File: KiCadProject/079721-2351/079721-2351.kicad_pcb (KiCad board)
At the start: 2 copper layers, 159.3 x 154.2 mm, 241 parts, among them IC1 HC244, IC101 uPC177C, IC201 MP493, IC401 D151811-0360, IC402 IS157, IC501 D151821-0020, IC601 MP5273, J201 Connected, J44 Conn_02x11_0x13_Top_Bottom_Sh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, J601 Connected, J711 Empty, Q802 C945, T1 2SB1015B, T211 RN1006, T711 2CS2001, T712A1 2SD1415, T721 2CS2001, T722A1 2SD1415, T751 CE1A3Q, T761 CE1A3Q, T801 2CS2001, T803 2CS4065, T811 2SC1815, T812 CE1A3Q, T821 Empty, T822 CE1A3Q (empty), T831 Empty, T832 CE1A3Q (empty), T841 2CS2001, T842 CE1A3Q, T851 Empty, T852 CE1A3Q (empty), T861 Empty, T911 RN1006, T921 RN1006, T921A1 Conn_01x01_Female, T921B1 Conn_01x01_Female, U1 4071, U2 4069, X601 Crystal

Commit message: Cleanup
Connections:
- net IC402_24 renamed IC401_24
- net Net-(C491-Pad2) renamed IC401_19
- net Vehicle_speed_sensor renamed Transsmision_control_module_2

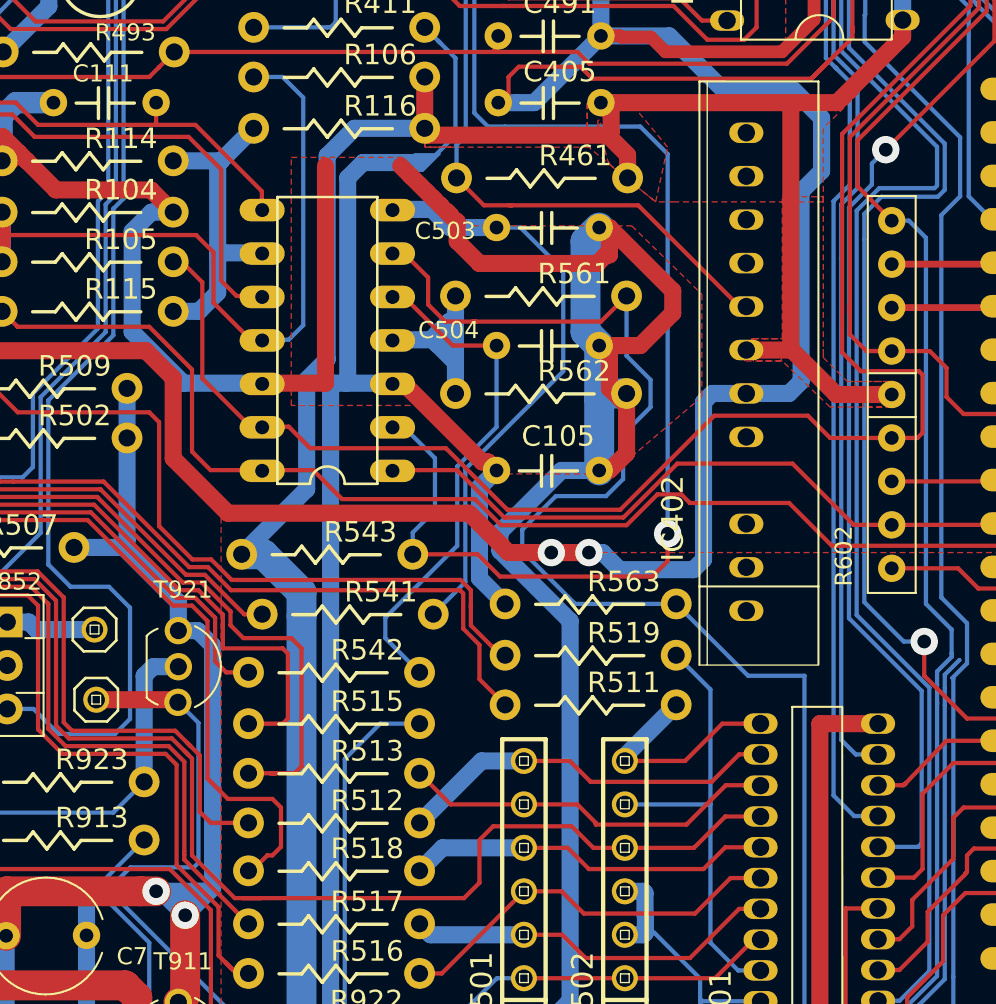
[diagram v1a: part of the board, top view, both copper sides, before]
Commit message: Cleanup
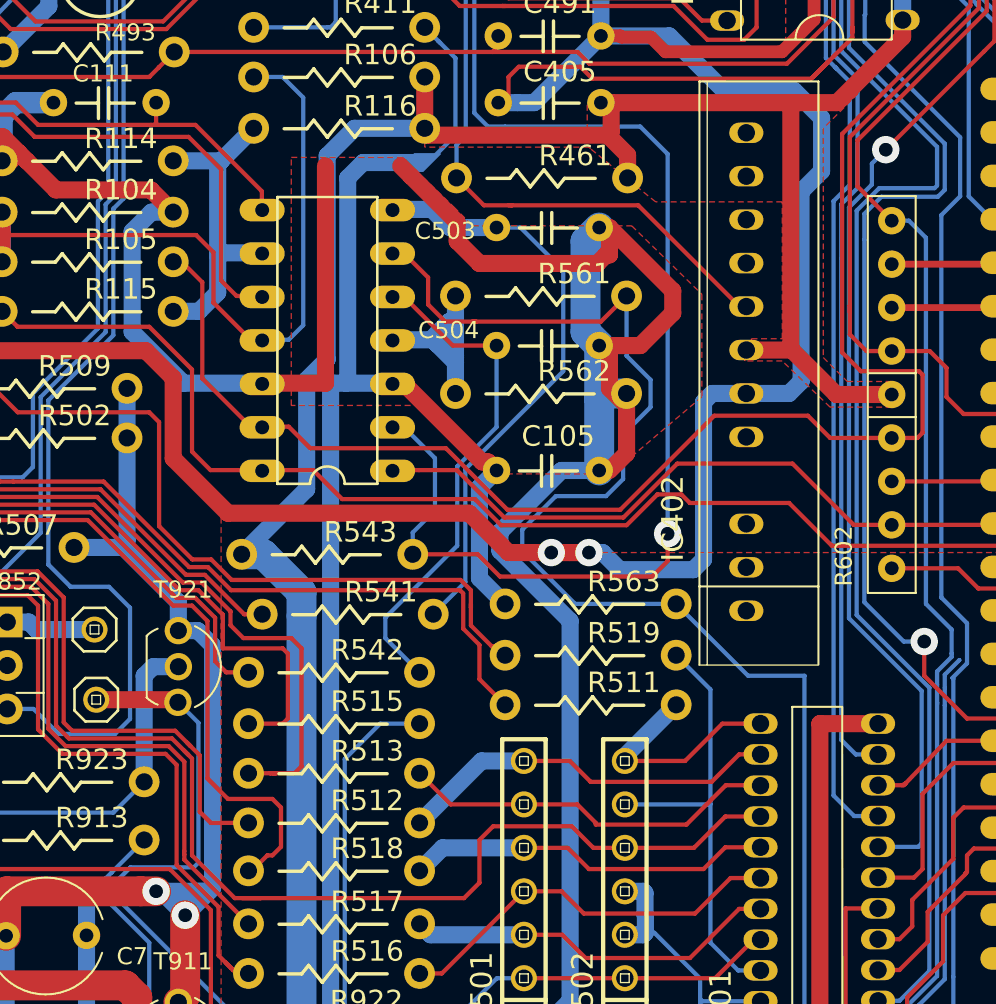
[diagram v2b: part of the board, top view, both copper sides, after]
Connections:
- net C501_2 renamed /IC501_20
- net C501_3 renamed /IC501_19
- net C501_5 renamed /IC501_17
- net C501_7 renamed /IC501_14
- net C502_7 renamed /IC501_13
- net IC101_2 renamed IC401_6
- net IC1_4 renamed +5V
- net IC201_15 renamed /IC201_15
- net IC201_16 renamed /IC201_16
- net IC201_18 renamed /IC201_18
- net IC201_19 renamed /IC201_19
- net IC401_19 renamed /IC401_19
- net IC402_4 renamed IC401_4
- net IC501_21 renamed /IC501_21
- net IC501_22 renamed /IC501_22
- net IC601_13 renamed /IC601_13
- net IC601_17 renamed /IC601_17
- net IC601_2 renamed /IC601_2
- net IC601_3 renamed /IC601_3
- net IC601_30 renamed /IC601_30
- net IC601_35 renamed /IC601_35
- net IC601_4 renamed /IC601_4
- net IC601_9 renamed /IC601_9
- net IC602_9 renamed Net-(U1-Pad12)
- net Net-(C201-Pad2) renamed /IC201_8
- net Net-(C202-Pad2) renamed /IC201_9
- net Net-(C203-Pad2) renamed /IC201_10
- net Net-(C204-Pad2) renamed /IC201_11
- net Net-(C401-Pad2) renamed /IC401_14
- net Net-(C422-Pad1) renamed /IC401_12
- net Net-(C432-Pad1) renamed /IC401_11
- net Net-(C442-Pad2) renamed /IC401_10
- net Net-(C452-Pad1) renamed /IC401_9
- net Net-(C472-Pad2) renamed /IC401_7
- net Net-(C481-Pad2) renamed /IC401_1
- net Net-(C501-Pad4) renamed /IC501_18
- net Net-(C501-Pad6) renamed /IC501_15
- net Net-(C502-Pad5) renamed /IC501_16
- net Net-(IC201-Pad4) renamed IC201_4
- net Net-(IC201-Pad7) renamed IC201_7
- net Net-(IC401-Pad13) renamed /IC401_13
- net Net-(IC601-Pad20) renamed /IC601_20
- net R412 renamed Net-(R411-Pad2)
- net R414 renamed Net-(C411-Pad1)
- net R432 renamed Water_thermosensor
- net R461_1 renamed /IC401_8
- IC401 pad 2: IC402_2 -> IC401_2
- IC402 pad 7: Net-(IC402-Pad7) -> IC402_2
- IC501 pad 7: IC402_2 -> IC401_2
- R461 pad 2: Net-(IC402-Pad7) -> IC402_2
- R462 pad 1: Net-(IC402-Pad7) -> IC402_2
- R463 pad 1: Net-(IC402-Pad7) -> IC402_2
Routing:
- net IC401_2: track 0.00 -> 99.3 mm, vias 0 -> 1
- net Net-(IC402-Pad7): track 63.6 -> 0.00 mm
- net IC402_2: track 99.3 -> 63.6 mm, vias 1 -> 0
